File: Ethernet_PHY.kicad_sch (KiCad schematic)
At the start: 16 parts, among them J7 RJ45_Hanrun_HR911105A_Horizon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, U4 LAN8720A, Y1 25MHz

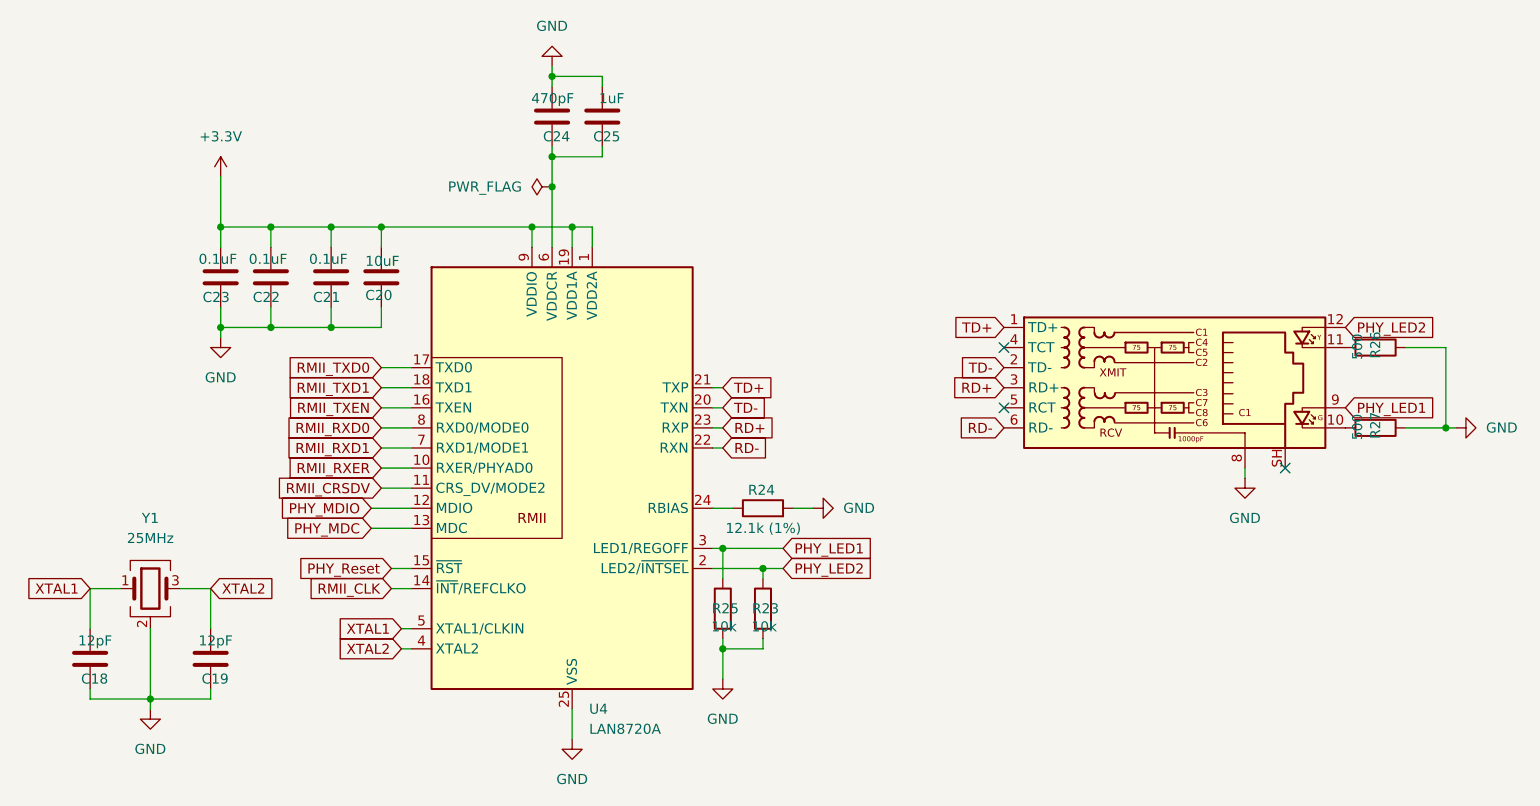
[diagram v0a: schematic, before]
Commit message: Updated
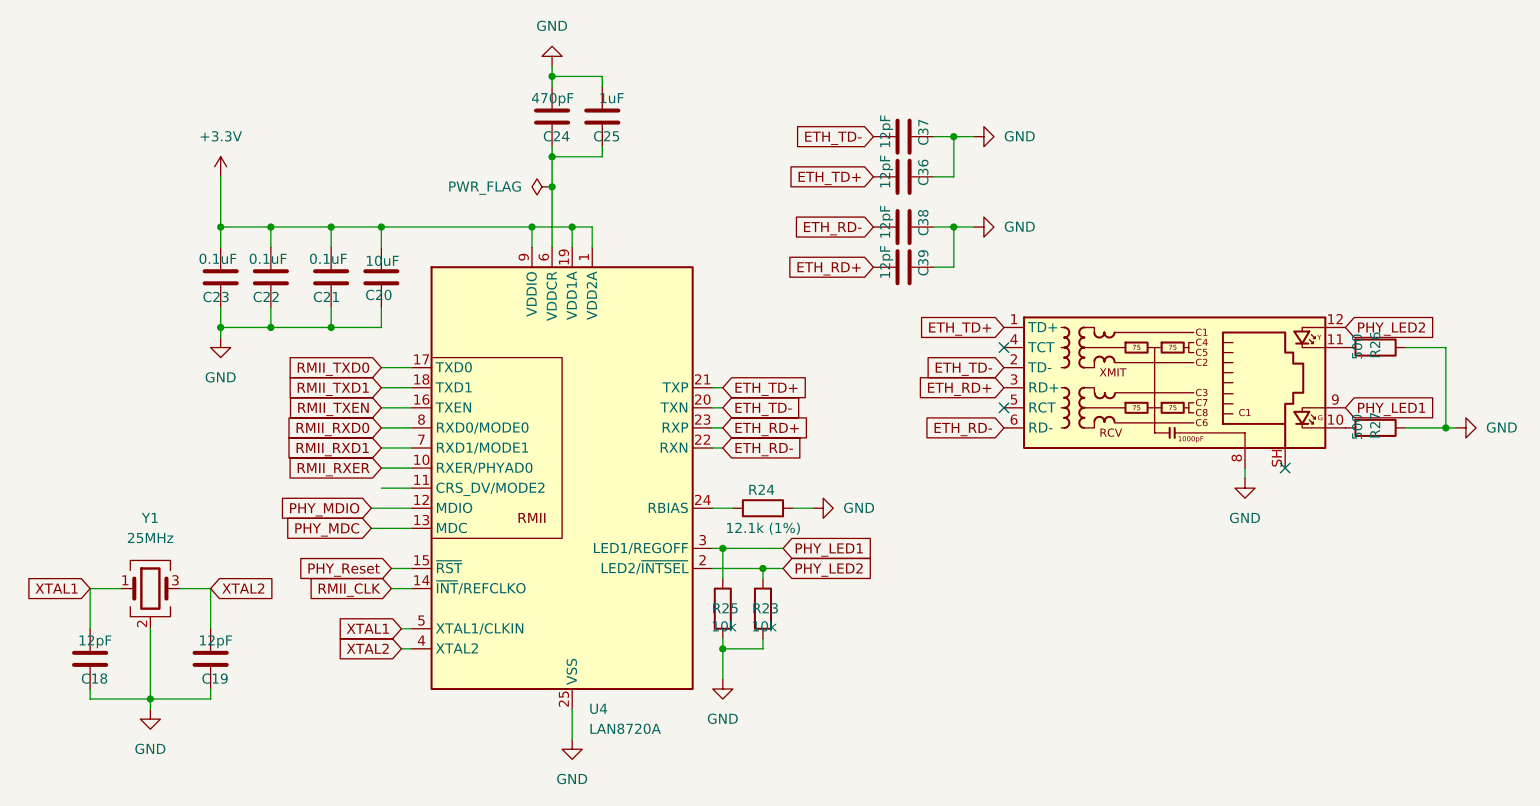
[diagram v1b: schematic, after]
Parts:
- added C36, C37, C38, C39: 12pF, Capacitor_SMD:C_0603_1608Metric, symbol Device:C
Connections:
- net GND: now also C36.1, C37.1, C38.1, C39.1
- net RD+ renamed ETH_RD+
- net ETH_RD+: now also C39.2
- net RD- renamed ETH_RD-
- net ETH_RD-: now also C38.2
- net RMII_CRSDV: no longer names the net of U4.11 (CRS_DV/MODE2)
- net TD+ renamed ETH_TD+
- net ETH_TD+: now also C36.2
- net TD- renamed ETH_TD-
- net ETH_TD-: now also C37.2
